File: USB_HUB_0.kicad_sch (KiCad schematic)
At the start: 30 parts, among them U1 VL822-QFN76, U2 W25Q32JVZPIQ, Y1 25Mhz

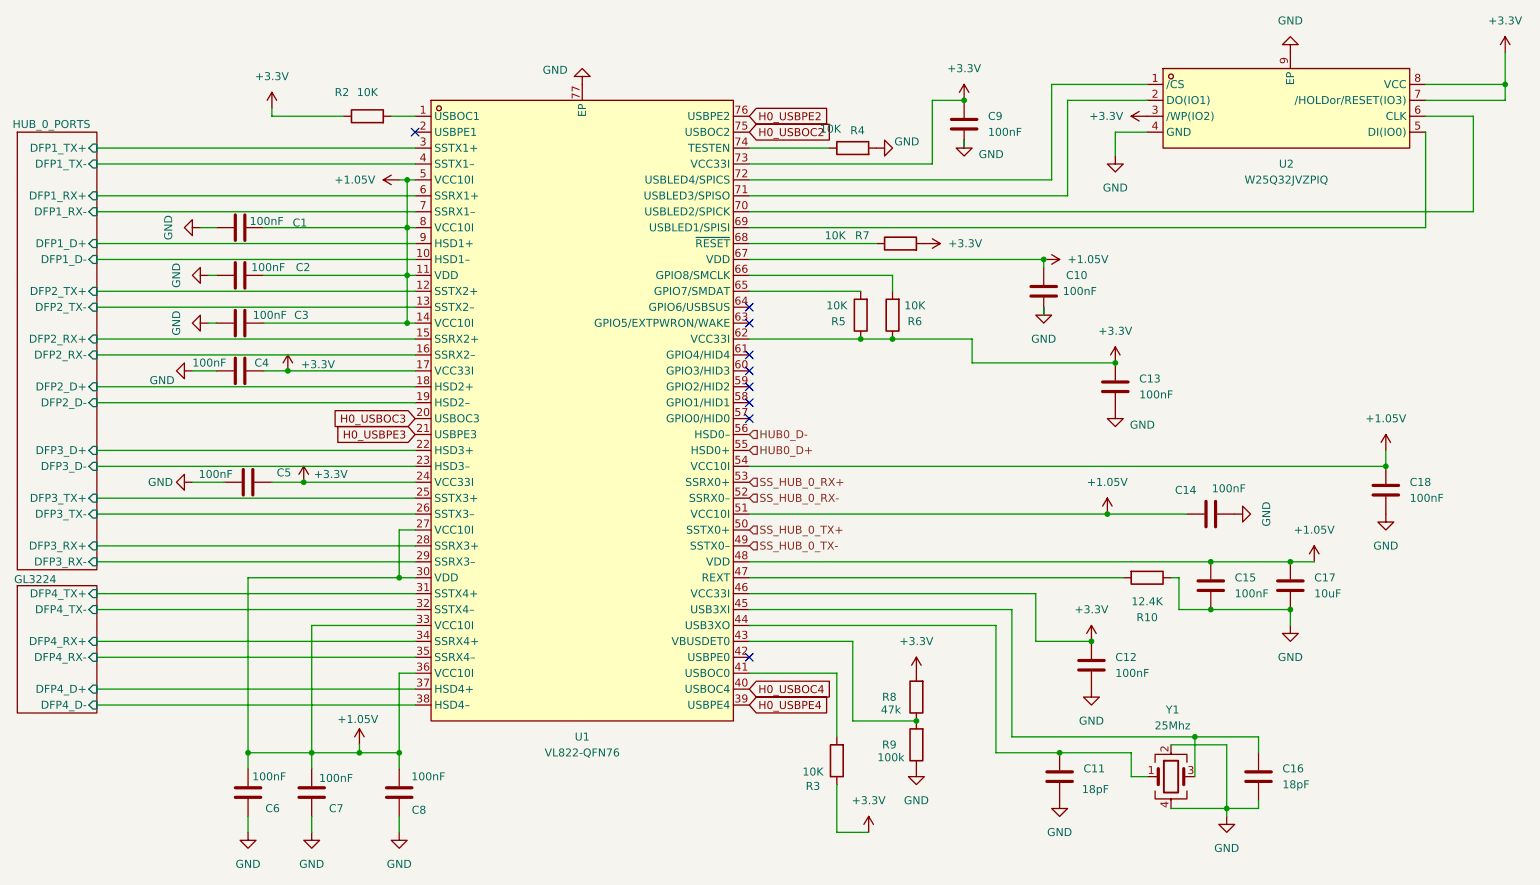
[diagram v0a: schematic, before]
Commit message: .
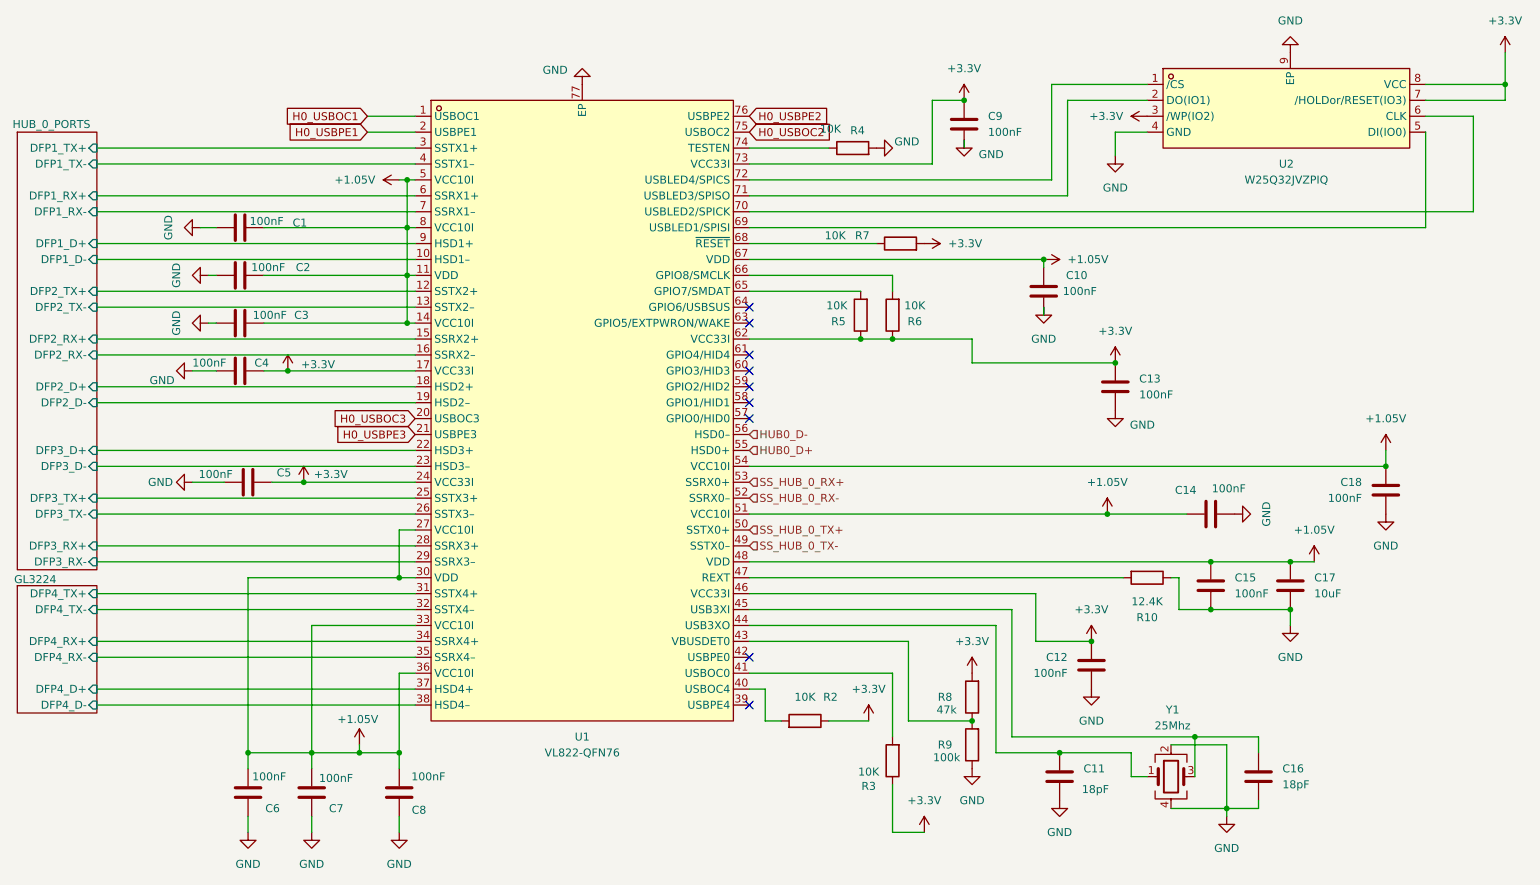
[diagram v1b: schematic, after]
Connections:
- net H0_USBOC4 is gone; now on an unnamed net: U1.40 (USBOC4)
- net at R2.2: no longer U1.1 (USBOC1)
- net H0_USBPE1: now reaches U1.2 (USBPE1)
- net H0_USBPE4: no longer names the net of U1.39 (USBPE4)
- new net H0_USBOC1: U1.1 (USBOC1)
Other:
- moved on the sheet: C12, R2, R3, R8, R9
